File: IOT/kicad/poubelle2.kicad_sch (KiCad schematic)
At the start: 3 parts

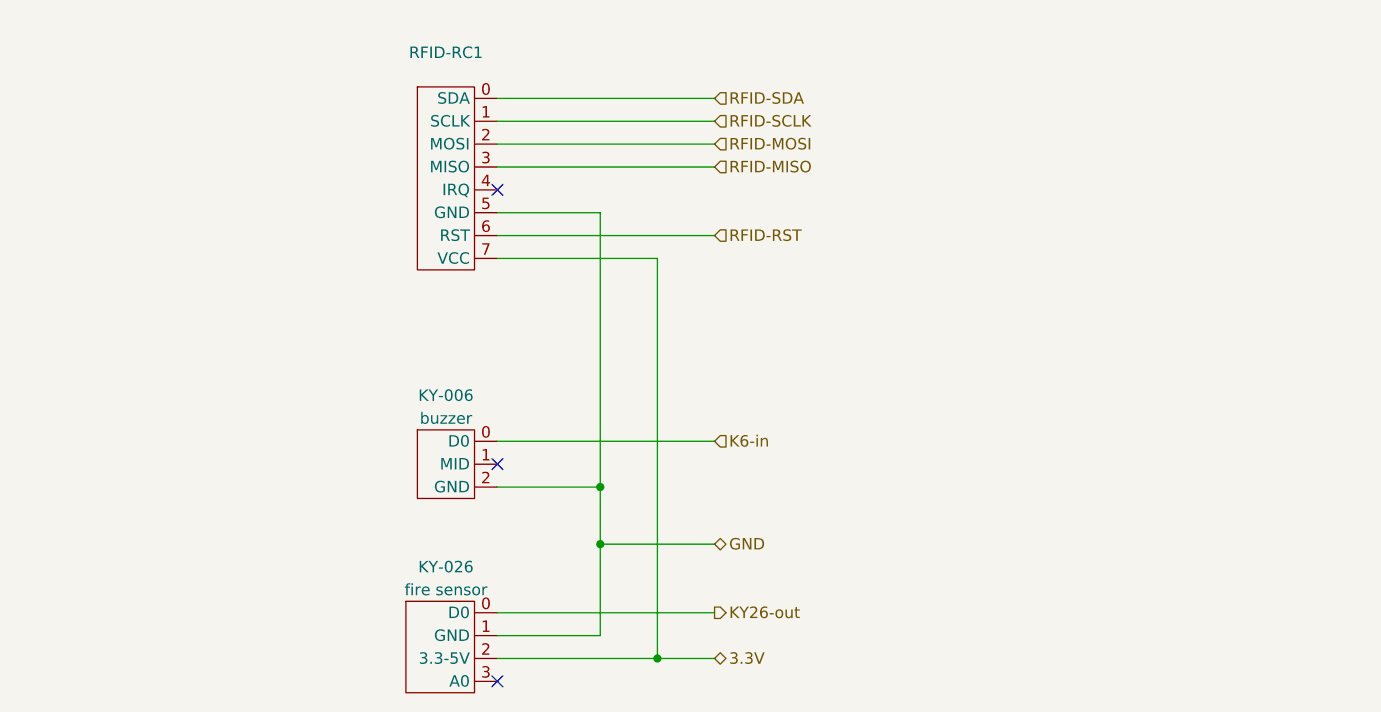
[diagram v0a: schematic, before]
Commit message: docs(iot): kicad filename + resistance + typo
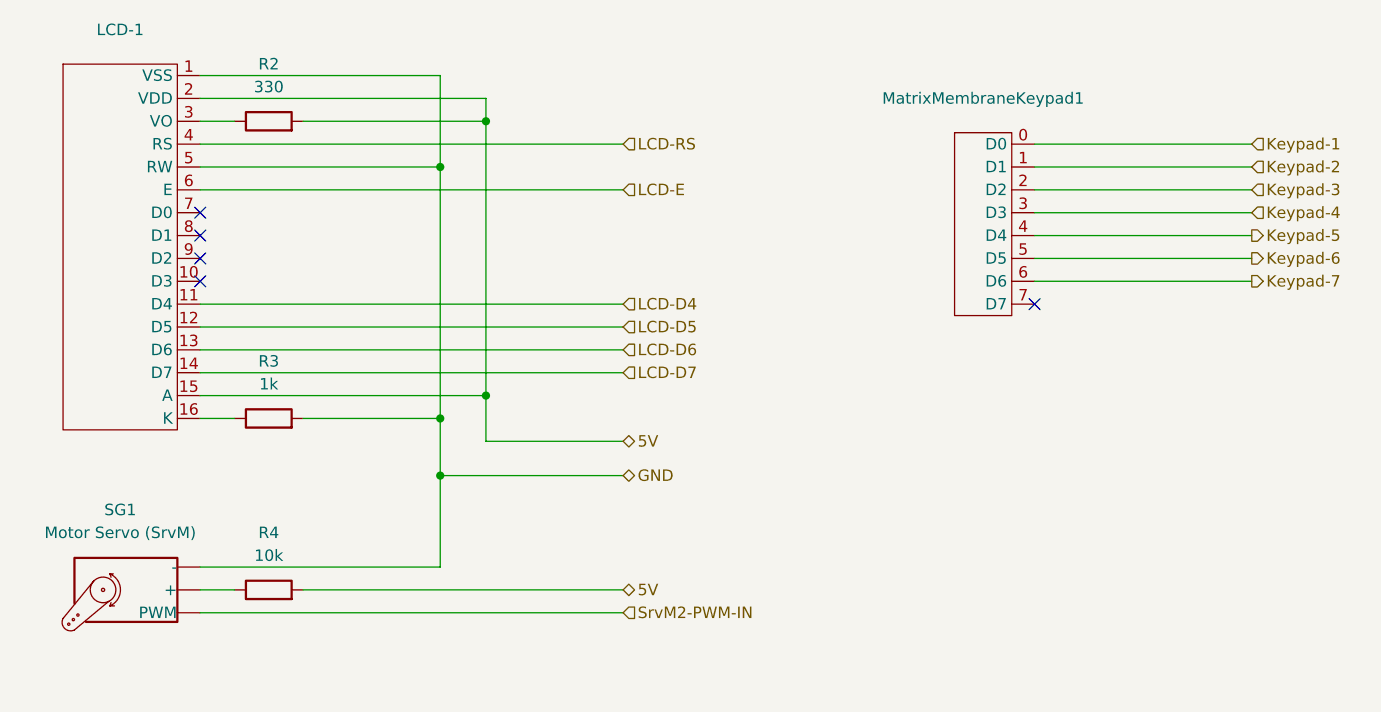
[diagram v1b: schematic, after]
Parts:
- removed KY-006: buzzer, symbol OrdureX:KY-006
- removed KY-026: fire sensor, symbol OrdureX:KY-026
- removed RFID-RC1: ~, symbol OrdureX:RFID-RC522
- added LCD-1: ~, symbol OrdureX:LCD-1602
- added MatrixMembraneKeypad1: ~, symbol OrdureX:27899
- added R2: 330, symbol Device:R
- added R3: 1k, symbol Device:R
- added R4: 10k, symbol Device:R
- added SG1: Motor Servo (SrvM), symbol Motor:Motor_Servo
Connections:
- net GND: now also LCD-1.1 (VSS), LCD-1.5 (RW), R3.2, SG1.3 (-)
- new net: LCD-1.16 (K), R3.1
- new net: R4.1, SG1.2 (+)
- new net: LCD-1.3 (VO), R2.1
- new net 5V: LCD-1.15 (A), LCD-1.2 (VDD), R2.2, R4.2
- new net Keypad-1: MatrixMembraneKeypad1.0 (D0)
- new net Keypad-2: MatrixMembraneKeypad1.1 (D1)
- new net Keypad-3: MatrixMembraneKeypad1.2 (D2)
- new net Keypad-4: MatrixMembraneKeypad1.3 (D3)
- new net Keypad-5: MatrixMembraneKeypad1.4 (D4)
- new net Keypad-6: MatrixMembraneKeypad1.5 (D5)
- new net Keypad-7: MatrixMembraneKeypad1.6 (D6)
- new net LCD-D4: LCD-1.11 (D4)
- new net LCD-D5: LCD-1.12 (D5)
- new net LCD-D6: LCD-1.13 (D6)
- new net LCD-D7: LCD-1.14 (D7)
- new net LCD-E: LCD-1.6 (E)
- new net LCD-RS: LCD-1.4 (RS)
- new net SrvM2-PWM-IN: SG1.1 (PWM)
- no-connect marks 3 -> 5
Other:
- title: Poubelle 1 -> Poubelle 2
